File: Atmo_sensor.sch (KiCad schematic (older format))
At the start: 1 part, among them J5 Conn_01x04_Female

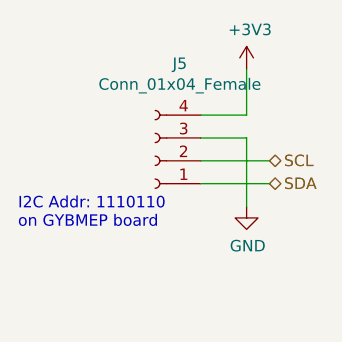
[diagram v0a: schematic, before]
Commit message: Finalize schematic
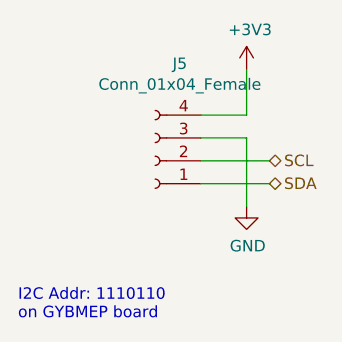
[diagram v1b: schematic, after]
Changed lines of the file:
@@
 Text HLabel 6100 3900 2    50   BiDi ~ 0
 SCL
-Text Notes 5000 4200 0    50   ~ 0
+Text Notes 5000 4600 0    50   ~ 0
 I2C Addr: 1110110\non GYBMEP board
 $Comp
